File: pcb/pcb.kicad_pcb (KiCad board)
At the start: 4 copper layers, 81.5 x 34 mm, 30 parts, among them J1 USB_C_Receptacle_USB2.0_16P, J3 Conn_01x02_MountingPin, J4 Conn_02x03_Odd_Even, SW1 SW_SPDT, SW2 RST, SW3 Kailh_Choc, SW4 Kailh_Choc, SW5 Kailh_Choc, SW6 Kailh_Choc, SW7 Kailh_Choc, SW8 Kailh_Choc, U1 nRF52840_holyiot_18010, U2 SRV05-4, U3 TP4056, U4 XC6206PxxxMR

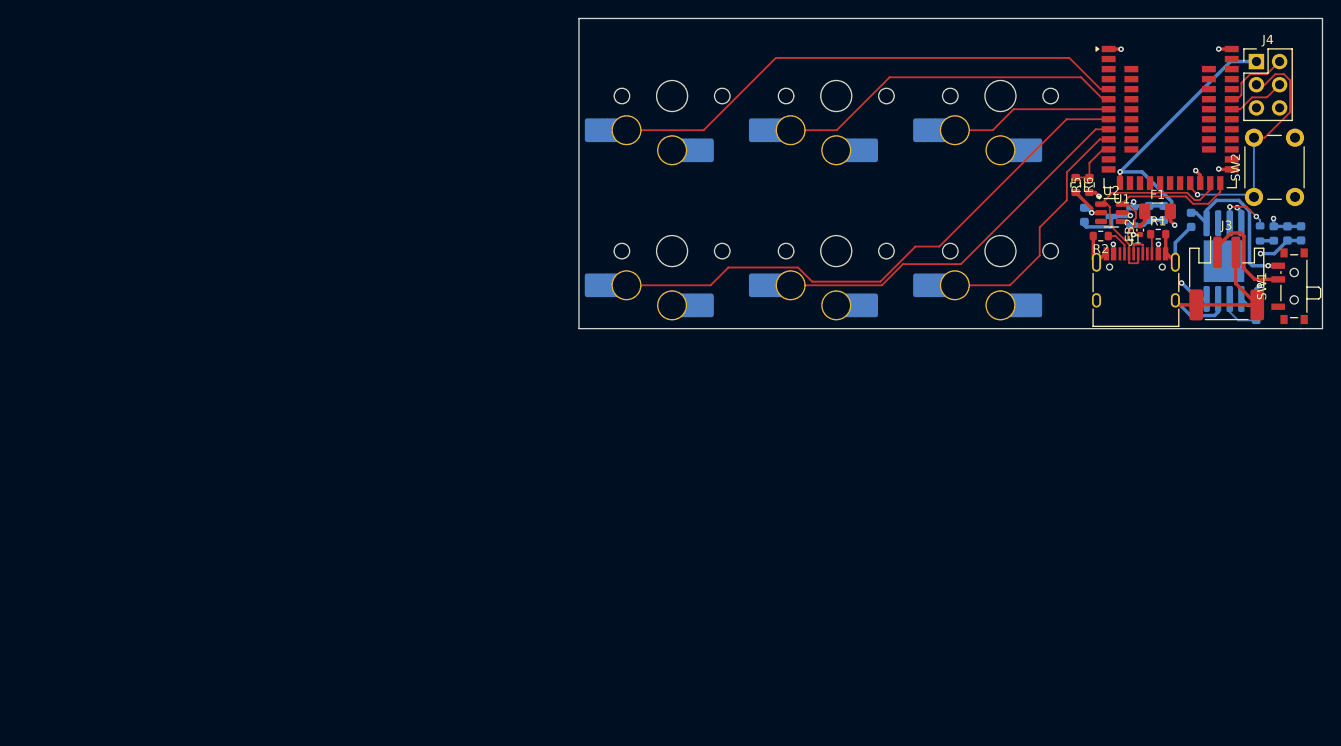
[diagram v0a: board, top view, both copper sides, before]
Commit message: pcb v3 - 2 layers again
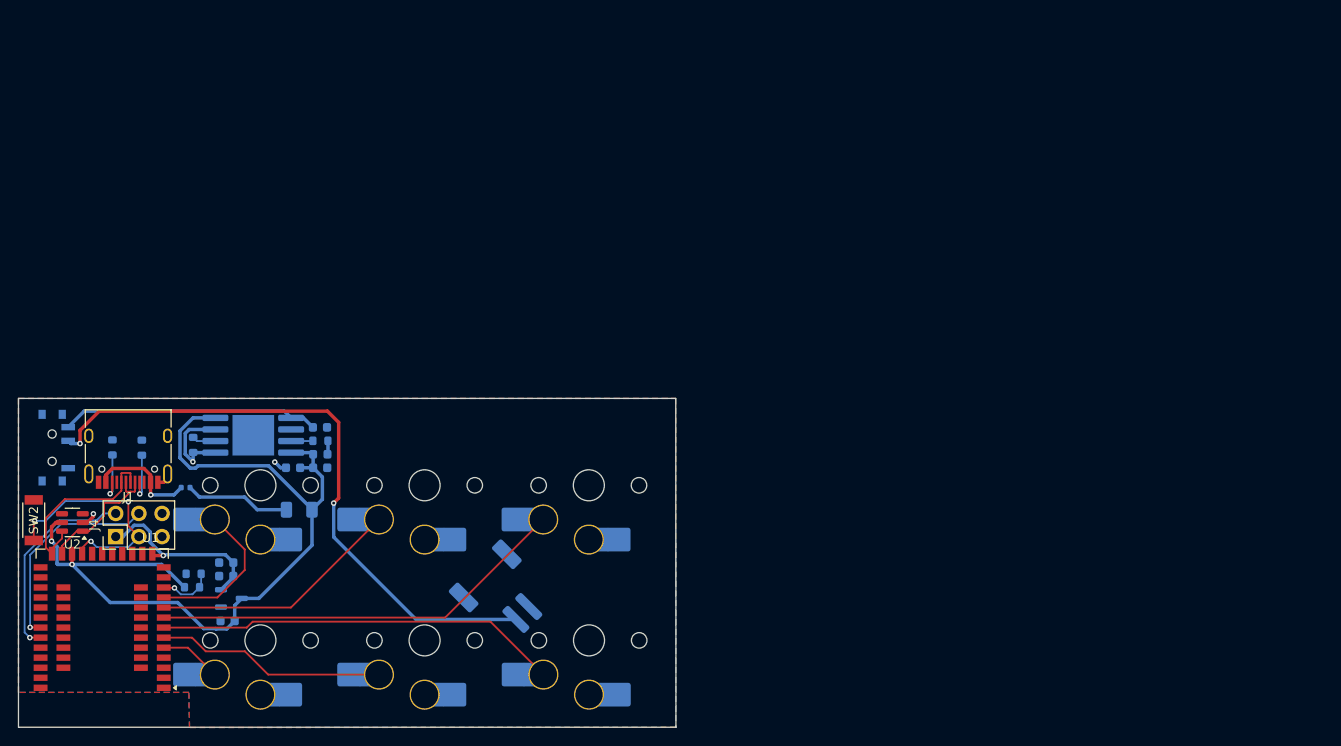
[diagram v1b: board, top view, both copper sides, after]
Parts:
- F1, FB2, J3, R1, R2, R5, R6, SW1: moved to B.Cu
- SW2: footprint Button_Switch_THT:SW_PUSH_6mm_H4.3mm -> horrortroll_lib:TS-1088R-02526
- moved SW2 138.4 mm to (30.4, 84.7)
- moved SW1 136.7 mm to (32.8, 76.8)
- moved J4 135.5 mm to (39.4, 86.5), turned to 90 degrees
- moved U1 130.9 mm to (37.9, 97.4), turned to 180 degrees
- moved U2 118.9 mm to (34.7, 85.0), turned to 180 degrees
- moved R4 117.4 mm to (47.9, 76.5), turned to -90 degrees
- moved R1 117.0 mm to (39.0, 76.7), turned to 90 degrees
- moved C3 112.0 mm to (58.9, 79.0), turned to 180 degrees
- moved J1 111.8 mm to (40.8, 76.5), turned to 180 degrees
- moved C2 110.6 mm to (61.8, 79.0), turned to 0 degrees
- moved C7 109.7 mm to (51.5, 89.3), turned to 180 degrees
- moved C6 108.7 mm to (51.5, 90.8), turned to 180 degrees
- moved FB2 108.4 mm to (47.1, 81.1), turned to 0 degrees
- moved U3 108.1 mm to (54.5, 75.4), turned to 0 degrees
- moved R5 107.8 mm to (47.8, 92.0), turned to 0 degrees
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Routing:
- net +5V: track 21.4 -> 95.2 mm, vias 7 -> 2
- net Net-(J3-Pin_1): track 12.1 -> 70.1 mm, vias 0 -> 2
- net /sw3: track 57.5 -> 6.82 mm
- net GND: track 58.3 -> 15.4 mm, vias 7 -> 3
- net /sw5: track 17.8 -> 44.3 mm
- net /SWDCLK: track 6.36 -> 22.9 mm, vias 0 -> 1
- net /sw6: track 61.7 -> 46.1 mm
- net /SWDIO: track 7.74 -> 22.3 mm, vias 0 -> 1
- net /sw7: track 41.9 -> 27.6 mm
- net +3.3V: track 34.3 -> 20.7 mm
- net /sw4: track 38.2 -> 25.3 mm
- net +BATT: track 18.2 -> 28.3 mm, vias 1 -> 0
- net /sw8: track 27.1 -> 17.0 mm
- net Net-(F1-Pad1): track 1.78 -> 11.6 mm
- net /USB-D-: track 24.1 -> 14.7 mm
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- added copper zone on B.Cu, net GND
- added copper zone on F.Cu, net GND
- removed copper zone on In2.Cu, net +5V
- removed copper zone on In1.Cu, net GND
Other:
- board size 81.5 x 34 mm -> 72.1 x 36.1 mm
- copper layers 4 -> 2
